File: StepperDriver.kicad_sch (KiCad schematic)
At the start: 18 parts, among them J701 WAGO 2065-100, J702 WAGO 2065-100, J703 WAGO 2065-100, J704 WAGO 2065-100, U701 TMC2130-LA

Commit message: Good Bye Imperial
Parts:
- C701: footprint V2_Capacitor_SMD:C_0603 -> V2_Capacitor_SMD:C_1608; symbol V2_Capacitor:0603_4u7 -> V2_Capacitor:1608_4u7
- C702: footprint V2_Capacitor_SMD:C_0603 -> V2_Capacitor_SMD:C_1608; symbol V2_Capacitor:0603_0u47 -> V2_Capacitor:1608_0u47
- C703, C705: footprint V2_Capacitor_SMD:C_0603 -> V2_Capacitor_SMD:C_1608; symbol V2_Capacitor:0603_0u1 -> V2_Capacitor:1608_0u1
- C707, C708: footprint V2_Capacitor_SMD:C_1210 -> V2_Capacitor_SMD:C_3225; symbol V2_Capacitor:1210_10u -> V2_Capacitor:3225_10u
- C709: footprint V2_Capacitor_SMD:C_0603 -> V2_Capacitor_SMD:C_1608; symbol V2_Capacitor:0603_0u022 -> V2_Capacitor:1608_0u022
- R701: footprint V2_Resistor_SMD:R_0603 -> V2_Resistor_SMD:R_1608; symbol V2_Resistor:0603_2R2 -> V2_Resistor:1608_2R2
- R702, R703: footprint V2_Resistor_SMD:R_0805 -> V2_Resistor_SMD:R_2012; symbol V2_Resistor:0805_0R11 -> V2_Resistor:2012_0R11
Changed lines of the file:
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@@
 	(title_block
 		(title "V2 drum")
-		(date "2026-04-14")
+		(date "2026-05-11")
 		(rev "2026-03-30")
 		(company "Versio Duo")
@@
 	)
 	(symbol
-		(lib_id "V2_Capacitor:1210_10u")
+		(lib_id "V2_Capacitor:3225_10u")
 		(at 158.75 49.53 0)
 		(unit 1)
@@
 			)
 		)
-		(property "Footprint" "V2_Capacitor_SMD:C_1210"
+		(property "Footprint" "V2_Capacitor_SMD:C_3225"
 			(at 158.75 66.548 0)
 			(hide yes)
@@
 	)
 	(symbol
-		(lib_id "V2_Capacitor:0603_4u7")
+		(lib_id "V2_Capacitor:1608_4u7")
 		(at 110.49 81.28 0)
 		(unit 1)
@@
 			)
 		)
-		(property "Footprint" "V2_Capacitor_SMD:C_0603"
+		(property "Footprint" "V2_Capacitor_SMD:C_1608"
 			(at 110.49 98.298 0)
 			(hide yes)
@@
 	)
 	(symbol
-		(lib_id "V2_Capacitor:0603_0u022")
+		(lib_id "V2_Capacitor:1608_0u022")
 		(at 175.26 91.44 0)
 		(unit 1)
@@
 			)
 		)
-		(property "Footprint" "V2_Capacitor_SMD:C_0603"
+		(property "Footprint" "V2_Capacitor_SMD:C_1608"
 			(at 175.26 108.458 0)
 			(hide yes)
@@
 	)
 	(symbol
-		(lib_id "V2_Capacitor:1210_10u")
+		(lib_id "V2_Capacitor:3225_10u")
 		(at 170.18 49.53 0)
 		(unit 1)
@@
 			)
 		)
-		(property "Footprint" "V2_Capacitor_SMD:C_1210"
+		(property "Footprint" "V2_Capacitor_SMD:C_3225"
 			(at 170.18 66.548 0)
 			(hide yes)
@@
 	)
 	(symbol
-		(lib_id "V2_Capacitor:0603_0u1")
+		(lib_id "V2_Capacitor:1608_0u1")
 		(at 124.46 49.53 0)
 		(unit 1)
@@
 			)
 		)
-		(property "Footprint" "V2_Capacitor_SMD:C_0603"
+		(property "Footprint" "V2_Capacitor_SMD:C_1608"
 			(at 124.46 66.548 0)
 			(hide yes)
@@
 	)
 	(symbol
-		(lib_id "V2_Resistor:0805_0R11")
+		(lib_id "V2_Resistor:2012_0R11")
 		(at 189.23 127 90)
 		(unit 1)
@@
 			)
 		)
-		(property "Footprint" "V2_Resistor_SMD:R_0805"
+		(property "Footprint" "V2_Resistor_SMD:R_2012"
 			(at 204.978 127 0)
 			(hide yes)
@@
 	)
 	(symbol
-		(lib_id "V2_Capacitor:0603_0u1")
+		(lib_id "V2_Capacitor:1608_0u1")
 		(at 139.7 86.36 0)
 		(unit 1)
@@
 			)
 		)
-		(property "Footprint" "V2_Capacitor_SMD:C_0603"
+		(property "Footprint" "V2_Capacitor_SMD:C_1608"
 			(at 139.7 103.378 0)
 			(hide yes)
@@
 	)
 	(symbol
-		(lib_id "V2_Resistor:0603_2R2")
+		(lib_id "V2_Resistor:1608_2R2")
 		(at 116.84 78.74 90)
 		(unit 1)
@@
 			)
 		)
-		(property "Footprint" "V2_Resistor_SMD:R_0603"
+		(property "Footprint" "V2_Resistor_SMD:R_1608"
 			(at 132.588 78.74 0)
 			(hide yes)
@@
 	)
 	(symbol
-		(lib_id "V2_Resistor:0805_0R11")
+		(lib_id "V2_Resistor:2012_0R11")
 		(at 189.23 129.54 90)
 		(unit 1)
@@
 			)
 		)
-		(property "Footprint" "V2_Resistor_SMD:R_0805"
+		(property "Footprint" "V2_Resistor_SMD:R_2012"
 			(at 204.978 129.54 0)
 			(hide yes)
@@
 	)
 	(symbol
-		(lib_id "V2_Capacitor:0603_0u47")
+		(lib_id "V2_Capacitor:1608_0u47")
 		(at 123.19 81.28 0)
 		(unit 1)
@@
 			)
 		)
-		(property "Footprint" "V2_Capacitor_SMD:C_0603"
+		(property "Footprint" "V2_Capacitor_SMD:C_1608"
 			(at 123.19 98.298 0)
 			(hide yes)

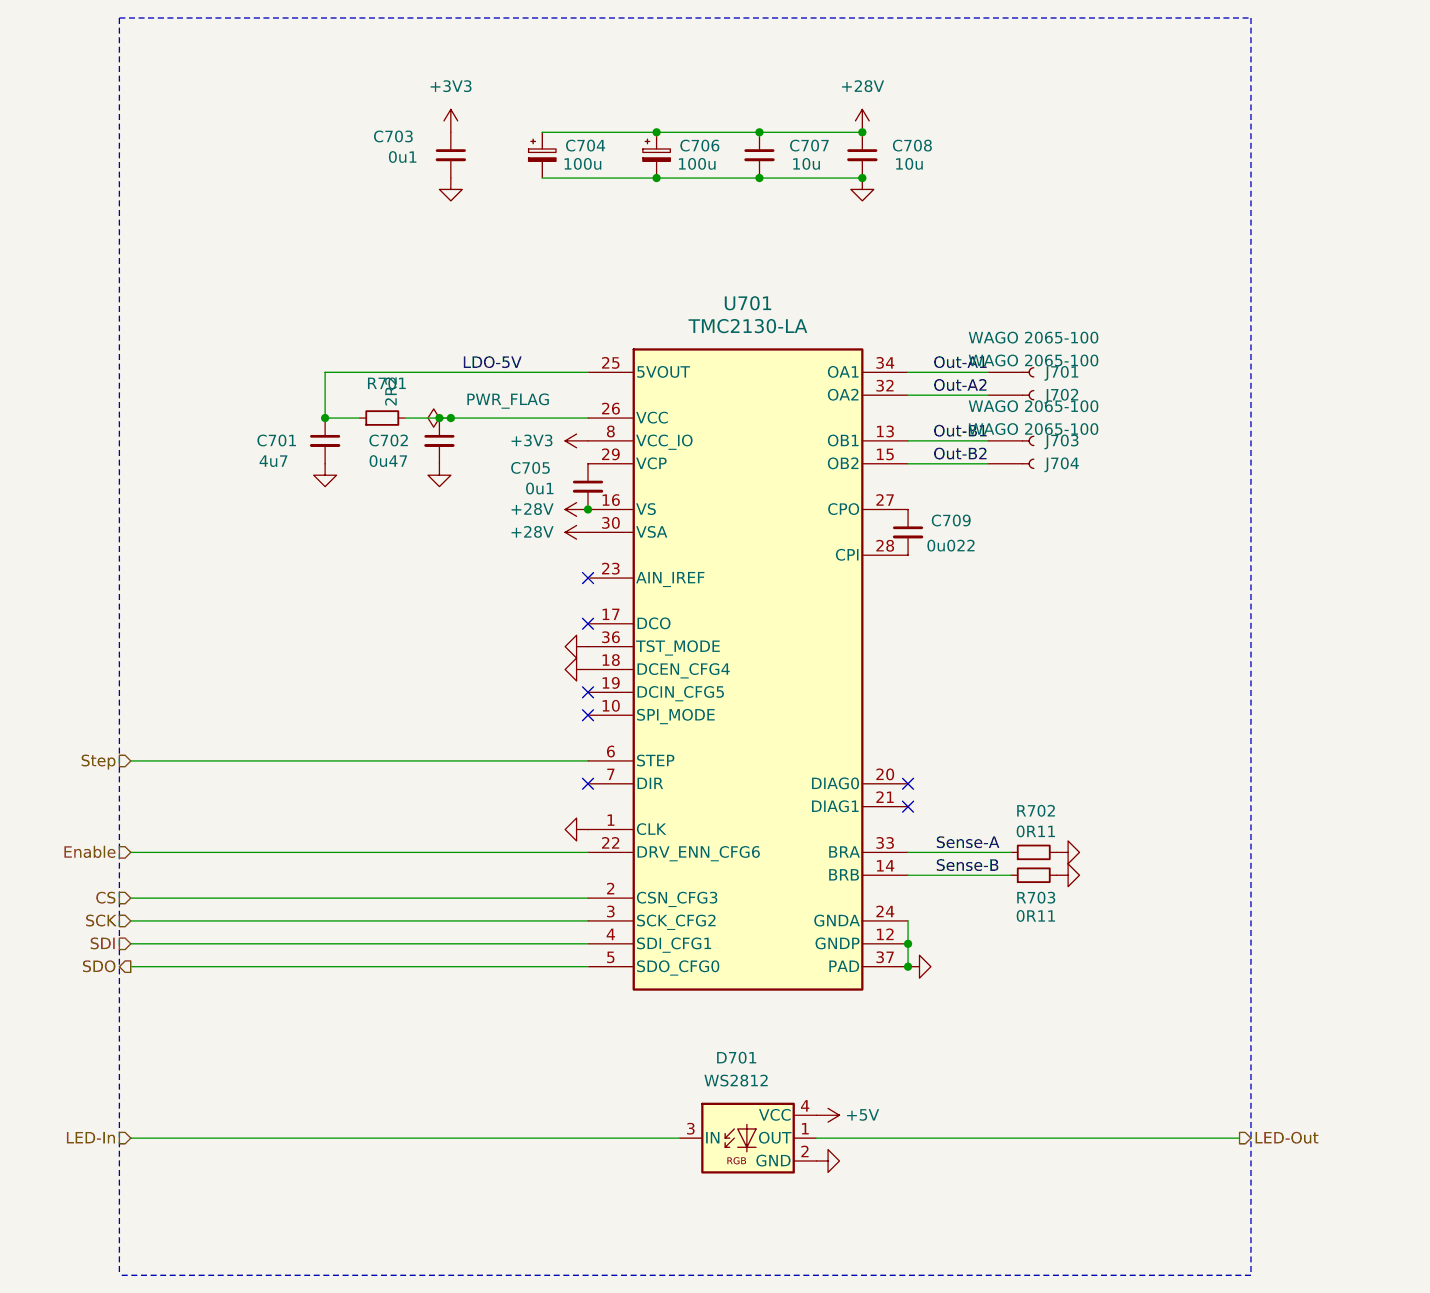
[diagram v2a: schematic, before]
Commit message: Refresh
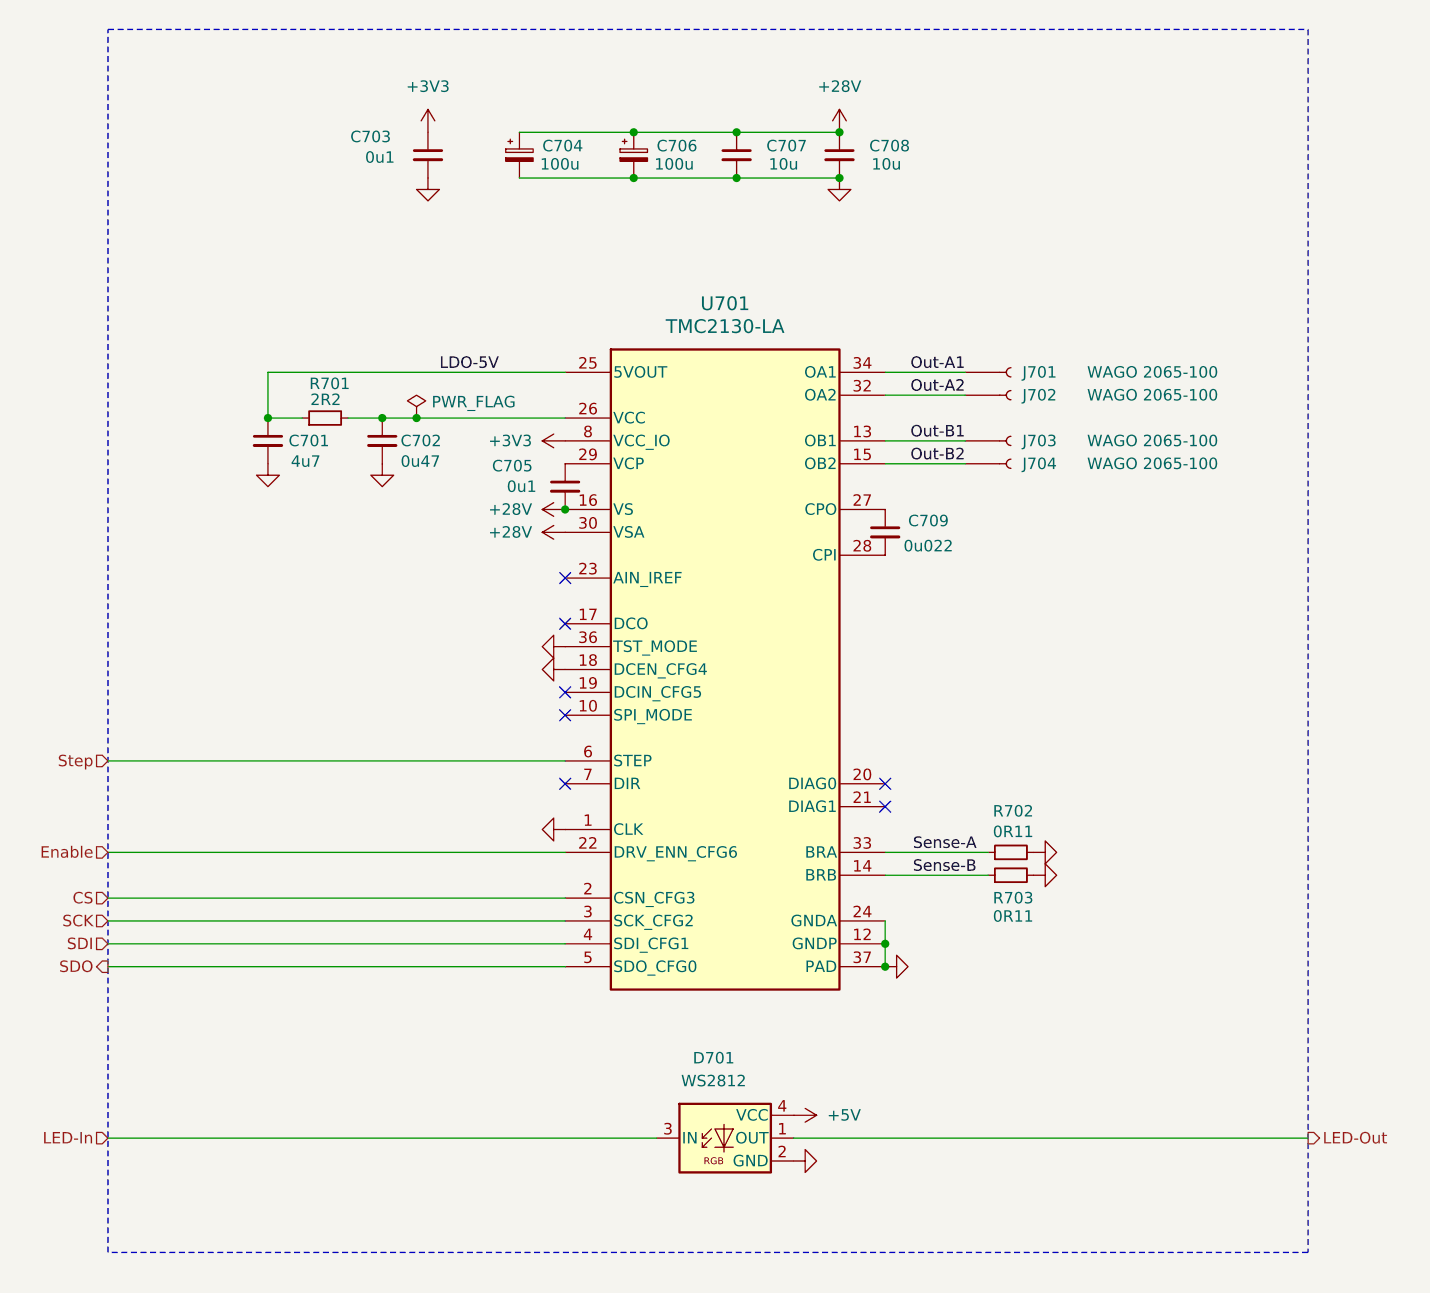
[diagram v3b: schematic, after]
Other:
- moved on the sheet: C701, C702, C703, C704, C705, C706, C707, C708, C709, D701, J701, J702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
